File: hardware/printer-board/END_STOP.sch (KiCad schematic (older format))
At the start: 19 parts, among them J15 X_MIN, J16 X_MAX, J17 Y_MIN, J18 Y_MAX, J19 Z_MIN, J20 Z_MAX, J45 END_SWITCH_DEBUG

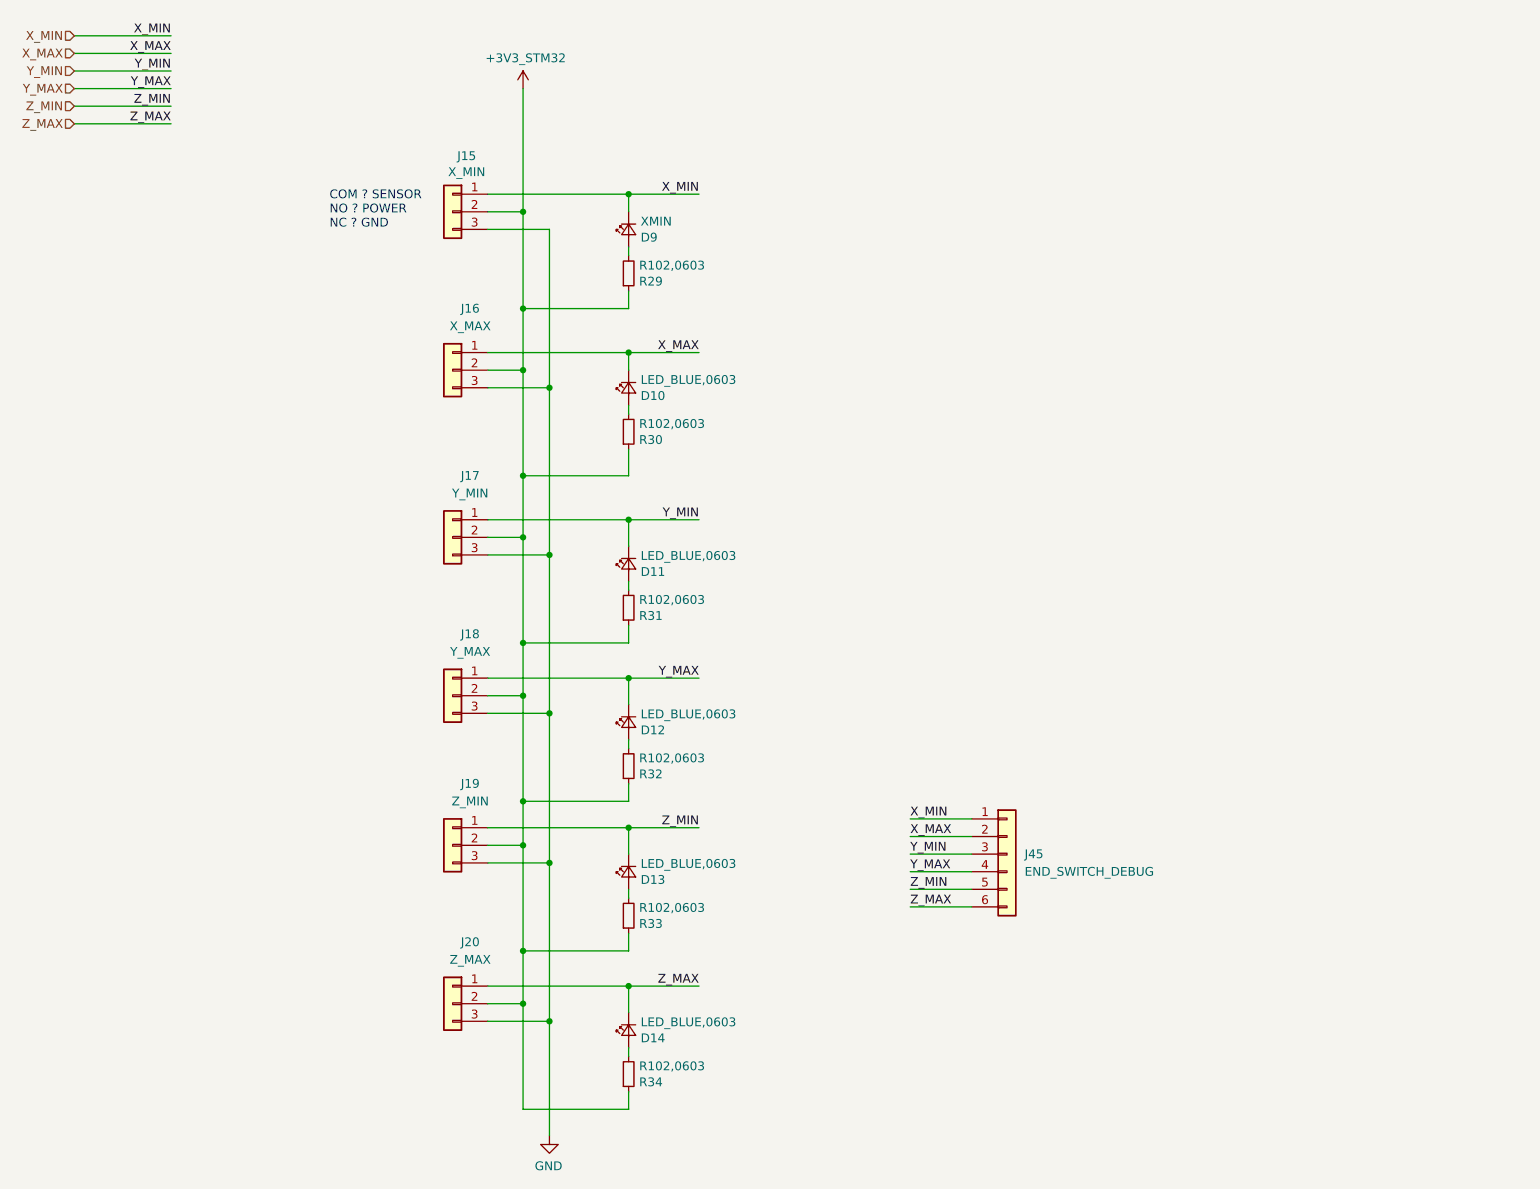
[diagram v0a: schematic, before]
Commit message: update,
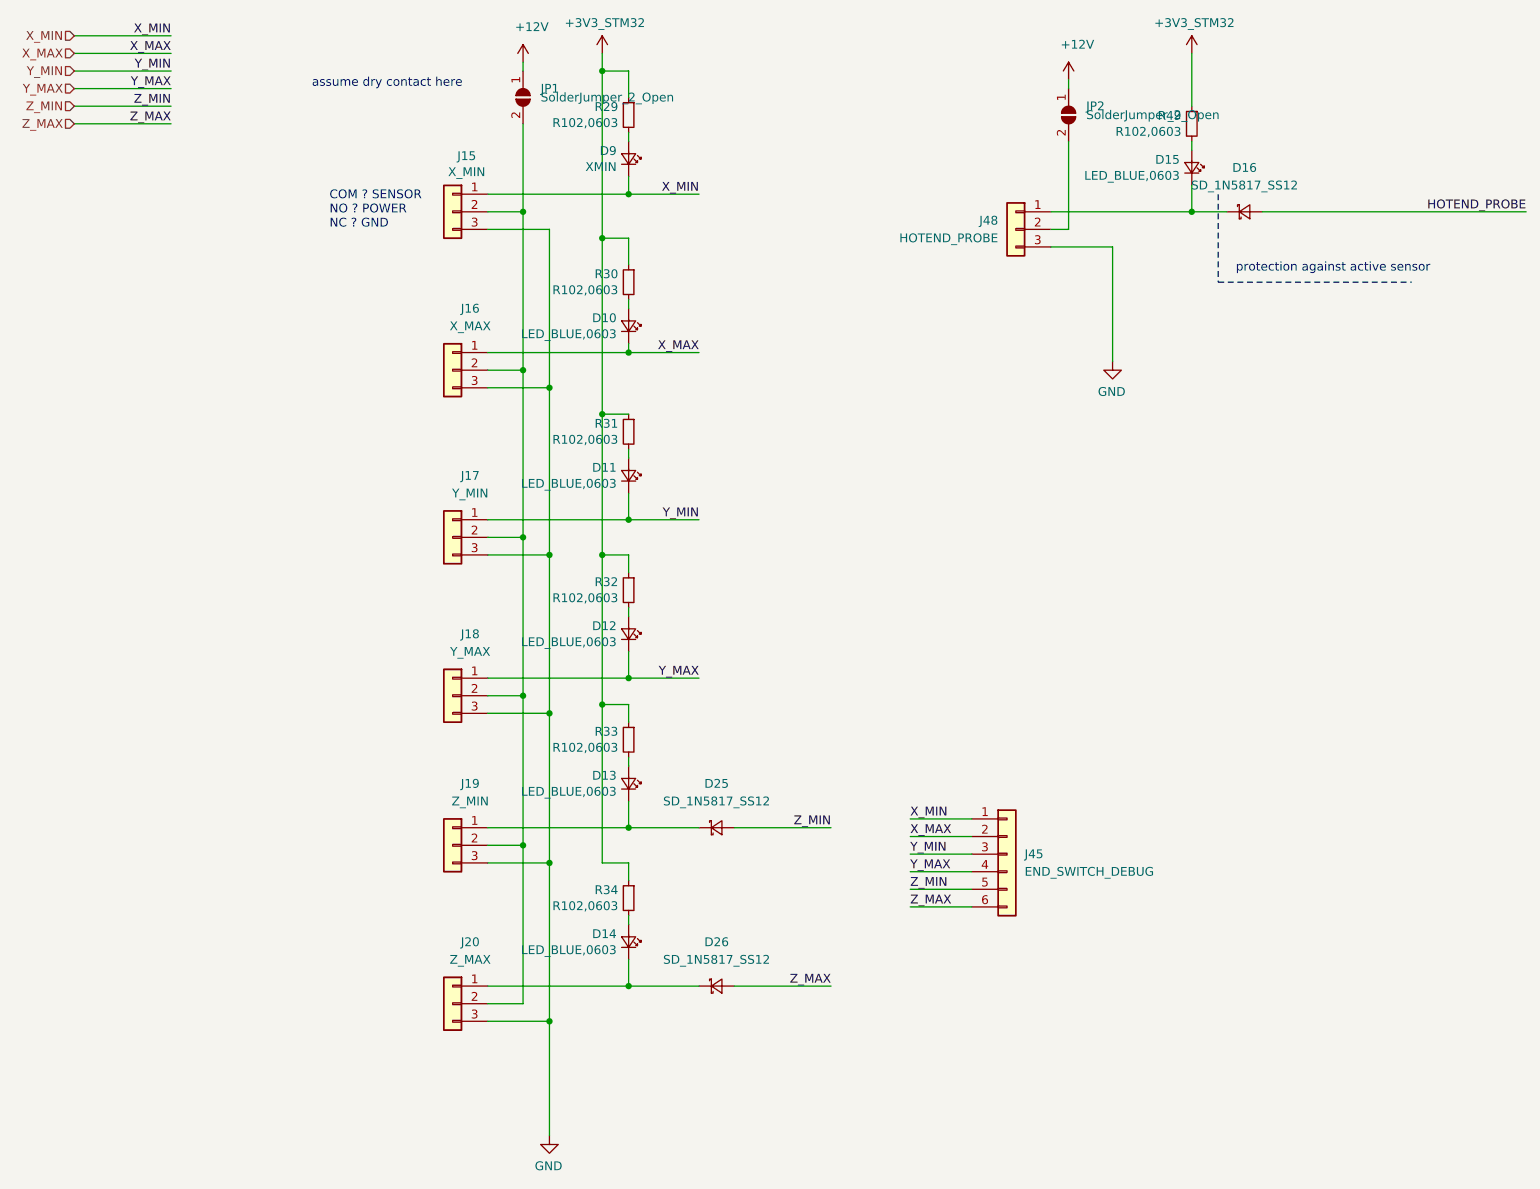
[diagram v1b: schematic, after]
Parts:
- added D15: LED_BLUE,0603, LED_SMD:LED_0603_1608Metric_Pad1.05x0.95mm_HandSolder, symbol taobao-led:LED_BLUE,0603
- added D16, D25, D26: SD_1N5817_SS12, symbol taobao-sd:SD_1N5817_SS12
- added J48: HOTEND_PROBE, footprint-lib:b3b-ph-kl,end_stop, symbol Connector_Generic:Conn_01x03
- added JP1, JP2: SolderJumper_2_Open, symbol Jumper:SolderJumper_2_Open
- added R49: R102,0603, Resistor_SMD:R_0603_1608Metric_Pad1.05x0.95mm_HandSolder, symbol taobao-r:R102,0603
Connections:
- net +3V3_STM32: now also R49.1; no longer J15.2 (Pin_2), J16.2 (Pin_2), J17.2 (Pin_2), J18.2 (Pin_2), J19.2 (Pin_2), J20.2 (Pin_2)
- net GND: now also J48.3 (Pin_3)
- net Z_MAX: now also D26.2 (A); no longer D14.1 (K), J20.1 (Pin_1)
- net Z_MIN: now also D25.2 (A); no longer D13.1 (K), J19.1 (Pin_1)
- new net: J15.2 (Pin_2), J16.2 (Pin_2), J17.2 (Pin_2), J18.2 (Pin_2), J19.2 (Pin_2), J20.2 (Pin_2), JP1.2 (B)
- new net: D13.1 (K), D25.1 (K), J19.1 (Pin_1)
- new net: D14.1 (K), D26.1 (K), J20.1 (Pin_1)
- new net: D15.1 (K), D16.1 (K), J48.1 (Pin_1)
- new net: J48.2 (Pin_2), JP2.2 (B)
- new net: D15.2 (A), R49.2
- new net +12V: JP1.1 (A), JP2.1 (A)
- new net HOTEND_PROBE: D16.2 (A)
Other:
- note added: "assume dry contact here"
- note added: "protection against active sensor"
- moved on the sheet: D10, D11, D12, D13, D14, D9, R29, R30, R31, R32, R33, R34
